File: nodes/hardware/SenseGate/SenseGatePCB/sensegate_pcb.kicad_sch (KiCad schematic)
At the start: 11 parts, among them J1 Conn_01x04_Socket, J2 Conn_01x04_Socket, J3 Conn_01x04_Socket, J4 Conn_01x24_Pin, J5 Conn_01x04_Socket, SW1 SW_Reed, SW2 SW_Reed, SW3 SW_Reed, U1 DD05CVSA

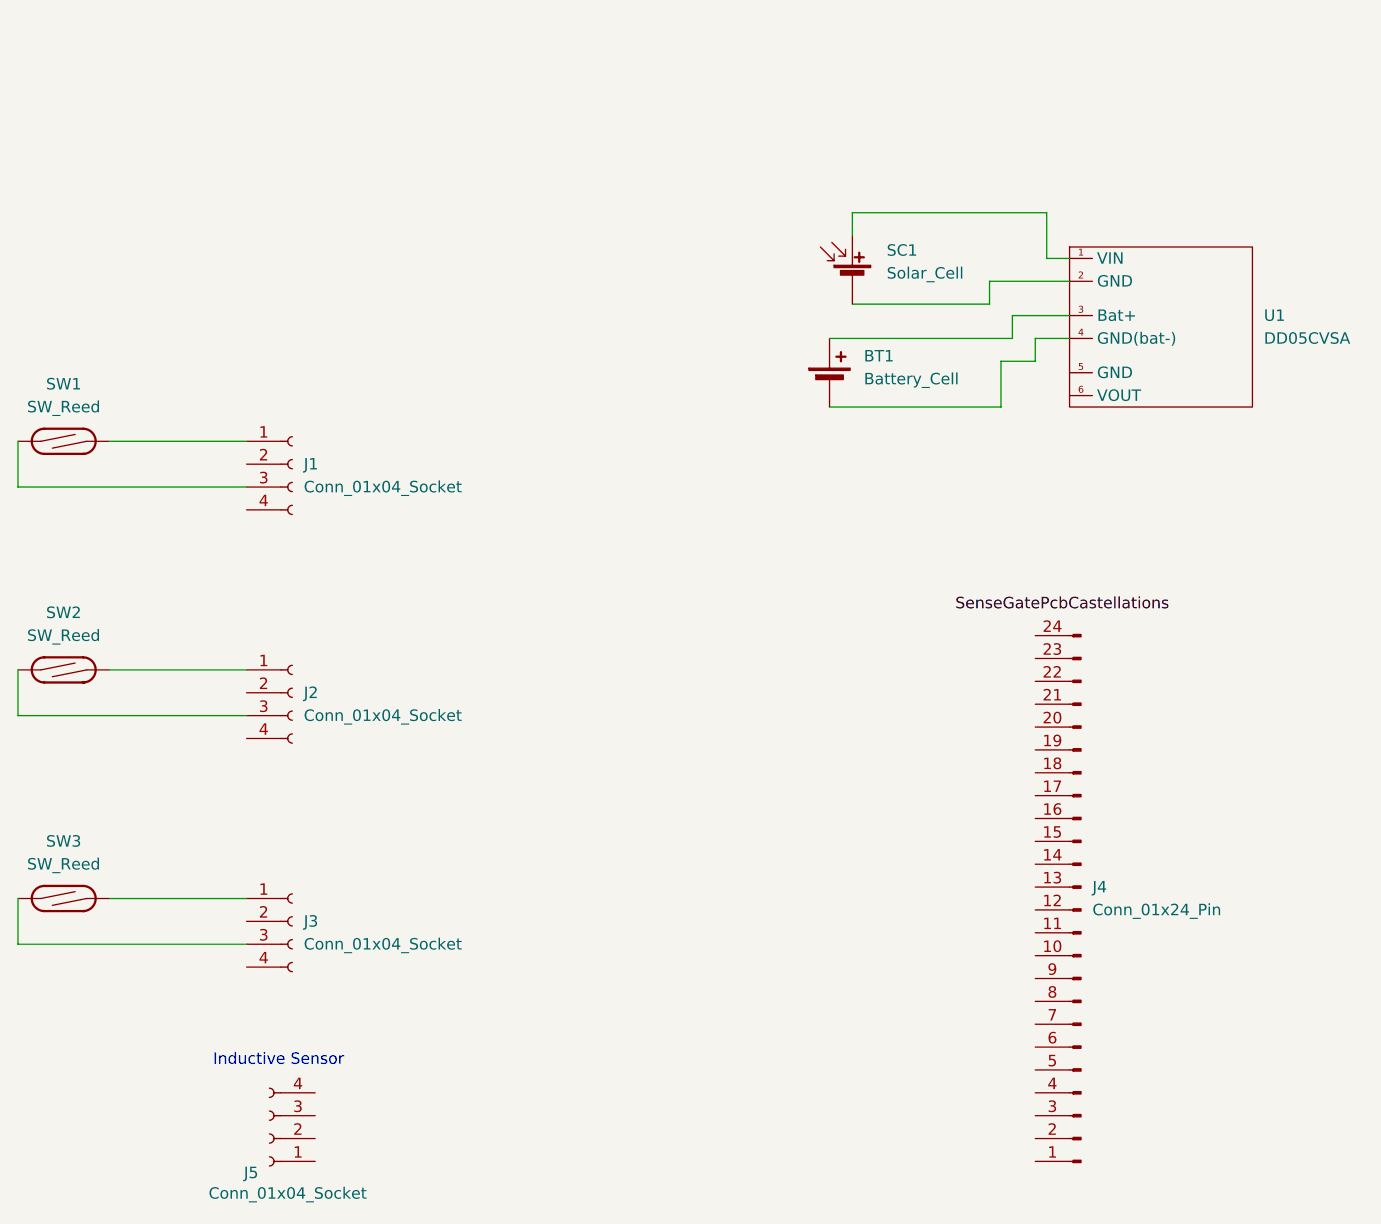
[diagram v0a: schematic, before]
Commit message: wip schematic and pcb
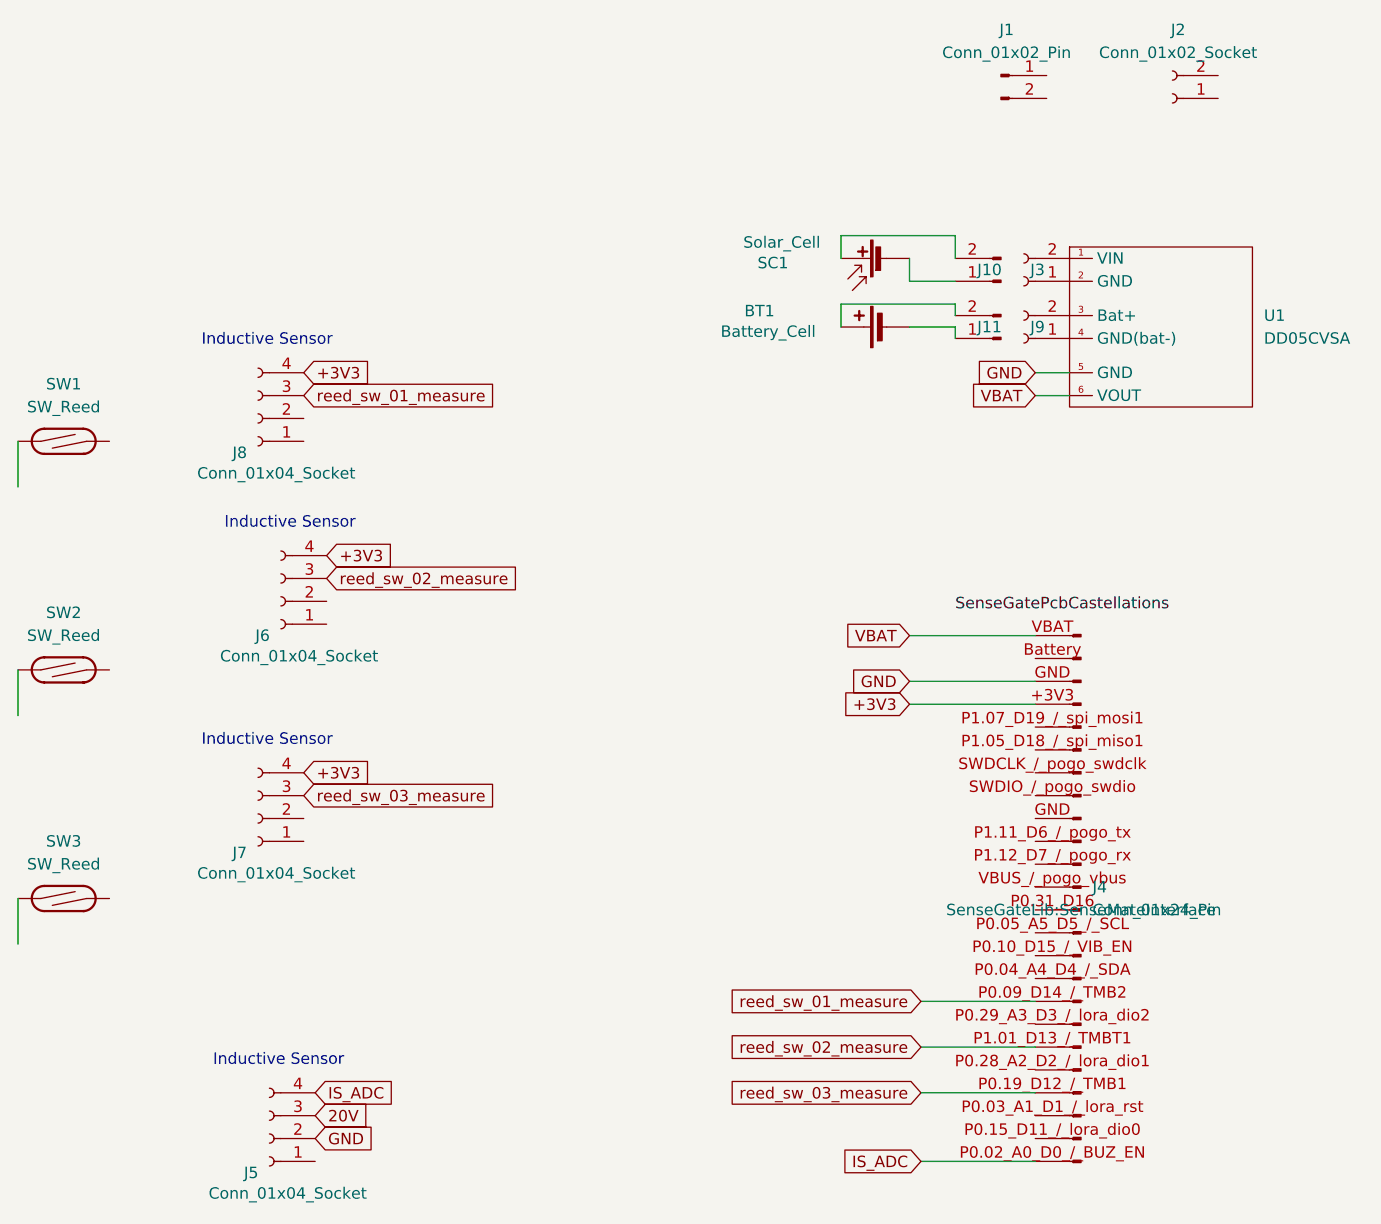
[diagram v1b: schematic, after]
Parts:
- removed J1, J2, J3: Conn_01x04_Socket, symbol Connector:Conn_01x04_Socket
- added J1, J10, J11: Conn_01x02_Pin, symbol Connector:Conn_01x02_Pin
- added J2, J3, J9: Conn_01x02_Socket, symbol Connector:Conn_01x02_Socket
- added J6, J7, J8: Conn_01x04_Socket, Connector_JST:JST_PH_B4B-PH-K_1x04_P2.00mm_Vertical, symbol Connector:Conn_01x04_Socket
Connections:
- net GND: now reaches J5.2 (Pin_2)
- net GND: now also J4.GND (Pin_22), U1.5 (GND)
- net 20V: now reaches J5.3 (Pin_3)
- net IS_ADC: now reaches J5.4 (Pin_4)
- net IS_ADC: now also J4.P0.02_A0_D0_/_BUZ_EN (Pin_1)
- net at SC1.1 (+): now also J10.2 (Pin_2); no longer U1.1 (VIN)
- net at SC1.2 (-): now also J10.1 (Pin_1); no longer U1.2 (GND)
- net at U1.3 (Bat+): now also J9.2 (Pin_2); no longer BT1.1 (+)
- net at U1.4 (GND(bat-)): now also J9.1 (Pin_1); no longer BT1.2 (-)
- net VBAT: now reaches U1.6 (VOUT)
- net VBAT: now also J4.VBAT (Pin_24)
- new net: J3.1 (Pin_1), U1.2 (GND)
- new net: J3.2 (Pin_2), U1.1 (VIN)
- new net: BT1.1 (+), J11.2 (Pin_2)
- new net: BT1.2 (-), J11.1 (Pin_1)
- new net +3V3: J4.+3V3 (Pin_21), J6.4 (Pin_4), J7.4 (Pin_4), J8.4 (Pin_4)
- new net reed_sw_01_measure: J4.P0.09_D14_/_TMB2 (Pin_8), J8.3 (Pin_3)
- new net reed_sw_02_measure: J4.P1.01_D13_/_TMBT1 (Pin_6), J6.3 (Pin_3)
- new net reed_sw_03_measure: J4.P0.19_D12_/_TMB1 (Pin_4), J7.3 (Pin_3)
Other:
- moved on the sheet: BT1, J4, SC1
